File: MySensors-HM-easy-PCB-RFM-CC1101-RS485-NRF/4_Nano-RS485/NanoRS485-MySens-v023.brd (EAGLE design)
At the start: 53 x 36 mm, 54 parts, among them IC1 ATSHA204A, IC2 AT25DF512C-SSHN-B, IC3 REG1117, IC31 ATMEGA168-TQFP, X2 1751264, Y2 8MHZ

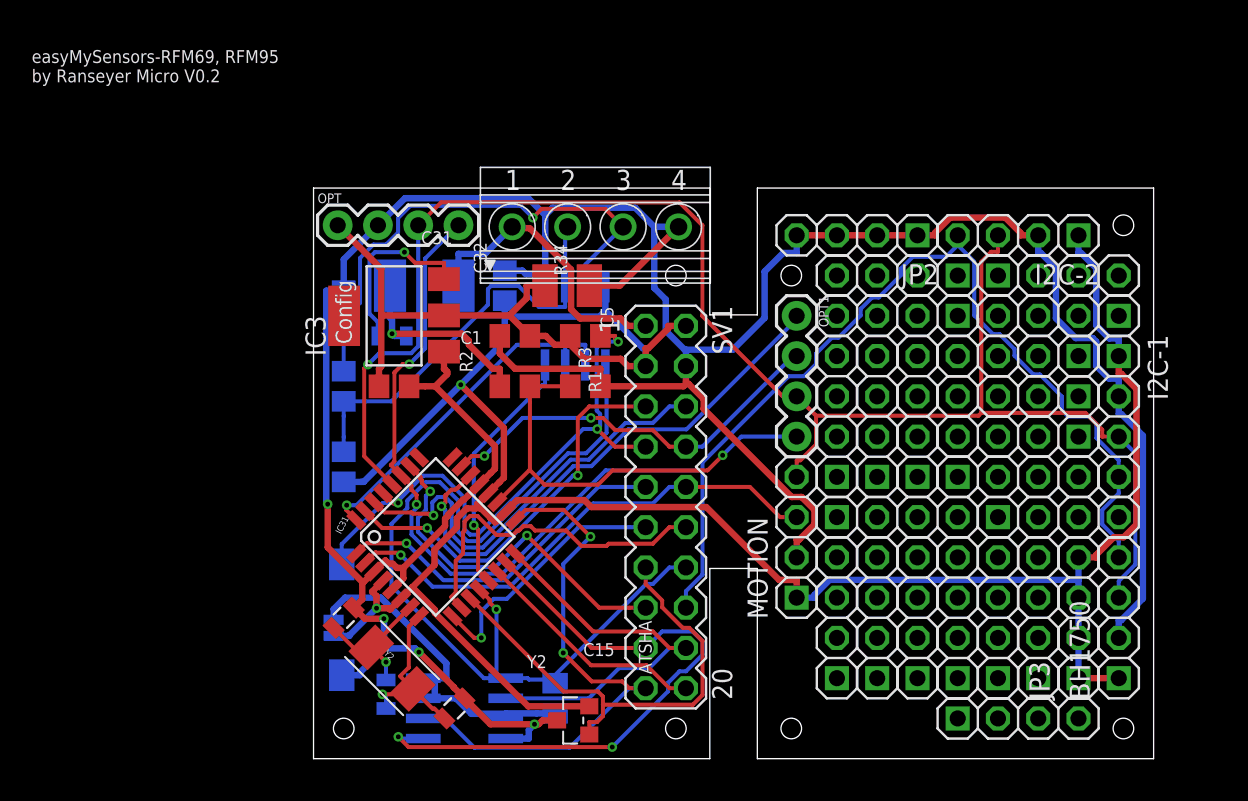
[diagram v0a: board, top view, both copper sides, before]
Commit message: Nano RS485
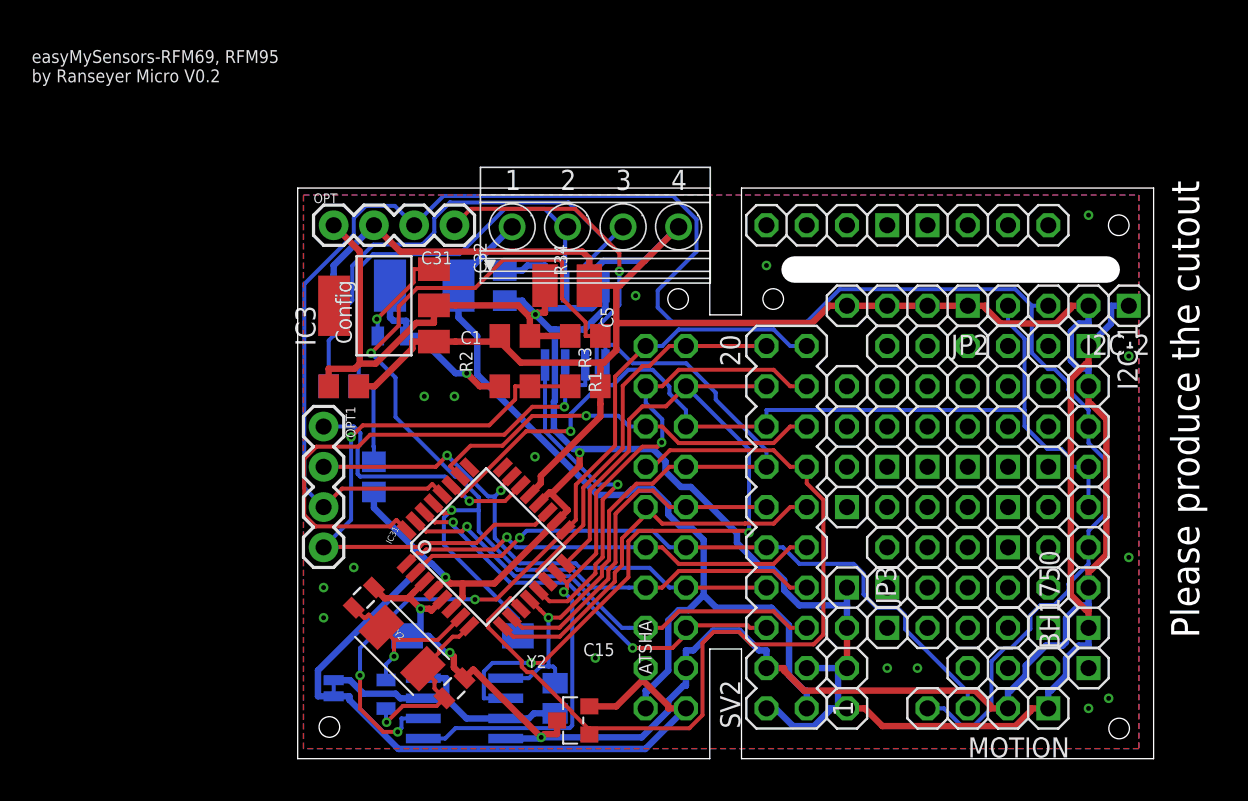
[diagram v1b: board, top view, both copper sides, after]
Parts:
- removed JP11, JP12, JP17, JP22, JP4, JP9: (no value), pinhead-2:1X04-S
- added SV2: (no value), con-lstb:MA10-2
- moved OPT1 30.7 mm to (0.64, 21.0)
- moved MOTION 16.2 mm to (42.5, 3.17), turned to 180 degrees
- moved JP16 15.7 mm to (32.4, 33.7)
- moved JP3 14.7 mm to (33.7, 6.99), turned to 270 degrees
- moved JP18 14.1 mm to (33.7, 19.7), turned to 90 degrees
- moved RESET 7.69 mm to (9.40, 7.75), turned to 180 degrees
- moved JP7 7.24 mm to (40.0, 8.26)
- moved JP23 7.24 mm to (40.0, 10.8), turned to 0 degrees
- moved JP19 6.54 mm to (46.4, 12.1)
- moved JP21 6.29 mm to (40.0, 13.3), turned to 180 degrees
- moved JP2 5.46 mm to (37.5, 28.6)
- moved JP13 5.46 mm to (41.3, 22.2), turned to 90 degrees
- moved I2C-2 5.46 mm to (47.6, 28.6)
- moved JP5 5.46 mm to (42.5, 33.7)
- moved JP1 3.81 mm to (1.27, 4.45)
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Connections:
- net A0: now also SV2.8
- net A3: now also SV2.15
- net A4: now also SV2.16
- net D1-TXD: now also SV2.5
- net D10_SS: now also SV2.20
- net D11_MOSI: now also SV2.17
- net D12_MISO: now also SV2.18
- net D13_SCK: now also SV2.19
- net D3: now also SV2.9
- net D4: now also SV2.10
- net D5: now also SV2.11
- net D6: now also SV2.12
- net D7-ATSHA: now also SV2.13
- net D8: now also SV2.14
- net GND: now also SV2.4
- net RESET: now also SV2.7
- net RXD: now also SV2.6
- net VCC: now also SV2.2, SV2.3
- net VIN: now also SV2.1
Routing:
- net VIN: track 18.6 -> 55.1 mm
- net RESET: track 37.7 -> 71.9 mm, vias 3 -> 2
- net D12_MISO: track 25.9 -> 56.0 mm, vias 0 -> 2
- net D7-ATSHA: track 30.3 -> 55.6 mm
- net A4: track 103.3 -> 80.6 mm
- net A5: track 101.7 -> 121.3 mm, vias 1 -> 0
- net VCC: track 184.0 -> 203.4 mm, vias 2 -> 3
- net A7: track 33.9 -> 16.6 mm
- net D8: track 59.1 -> 44.5 mm
- net D13_SCK: track 36.2 -> 49.9 mm, vias 2 -> 3
- net D2_INT0: track 23.0 -> 33.7 mm
- net D4: track 31.8 -> 42.5 mm
- net D10_SS: track 14.9 -> 25.0 mm
- net A0: track 25.5 -> 34.9 mm
- net A6: track 29.2 -> 38.4 mm
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- added copper zone on layer 1, net GND
- added copper zone on layer 16, net GND
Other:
- board size 53 x 36 mm -> 54 x 36 mm
- board text added: "Please produce the cutout"
